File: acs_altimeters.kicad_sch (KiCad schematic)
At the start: 15 parts, among them U4 BMP581, U5 BMP581, U6 BMP581

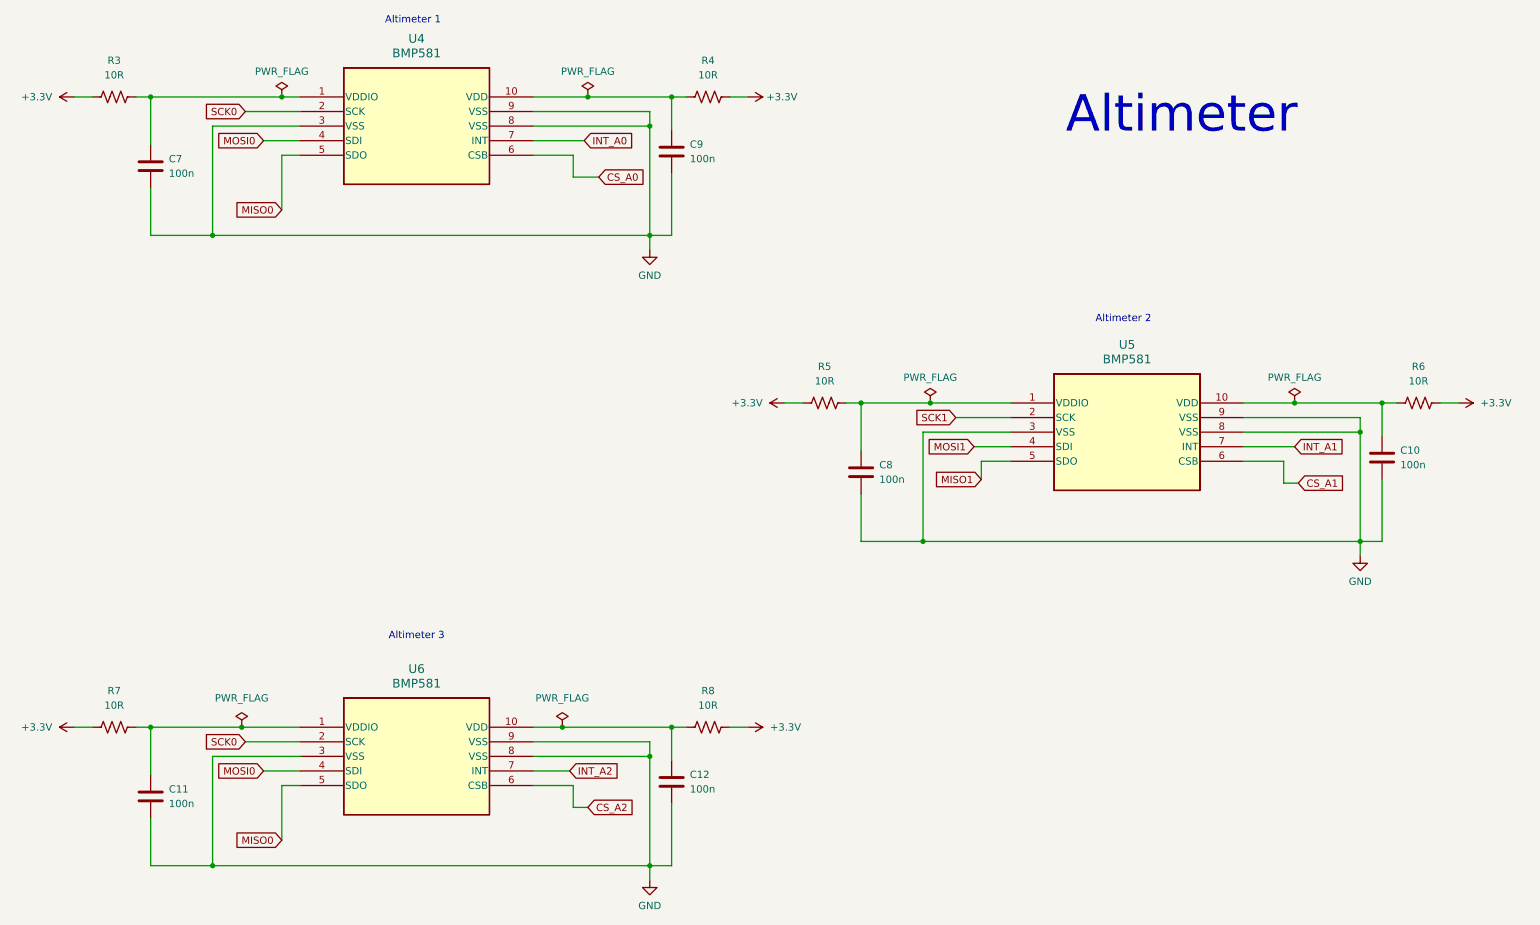
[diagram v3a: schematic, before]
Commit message: miso-mosi-fix
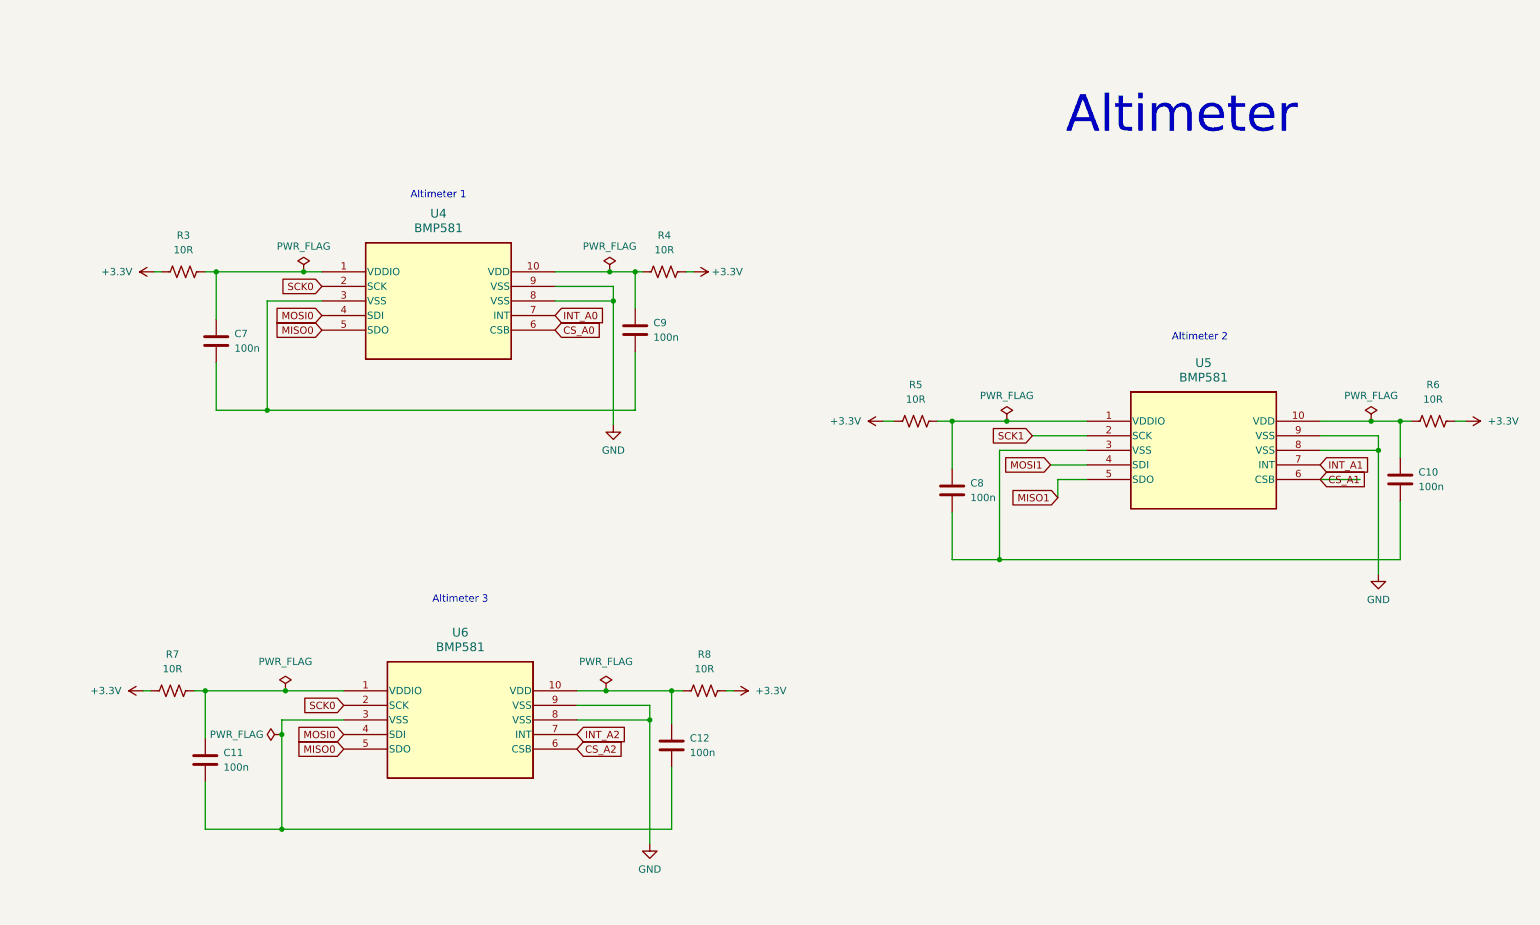
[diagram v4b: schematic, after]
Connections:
- net GND: no longer C10.1, C11.2, C12.1, C7.2, C8.2, C9.1, U4.3 (VSS), U5.3 (VSS), U6.3 (VSS)
- new net: C7.2, C9.1, U4.3 (VSS)
- new net: C10.1, C8.2, U5.3 (VSS)
- new net: C11.2, C12.1, U6.3 (VSS)
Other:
- moved on the sheet: C10, C11, C12, C7, C8, C9, R3, R4, R5, R6, R7, R8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
